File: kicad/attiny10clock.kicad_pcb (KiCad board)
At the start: 2 copper layers, 71 x 37 mm, 41 parts, among them J1 USB_B_Micro, J2 Conn_02x04_Odd_Even, SW1 SW_DIP_x01, SW2 SW_DIP_x01, SW3 SW_DIP_x01, SW4 SW_DIP_x01, SW5 SW_DIP_x01, U1 ATtiny10-TS, U2 NPIC6C595, U3 NPIC6C595, U4 NPIC6C595, U5 NPIC6C595, U6 RT8097AHGB, X1 DFA-S15

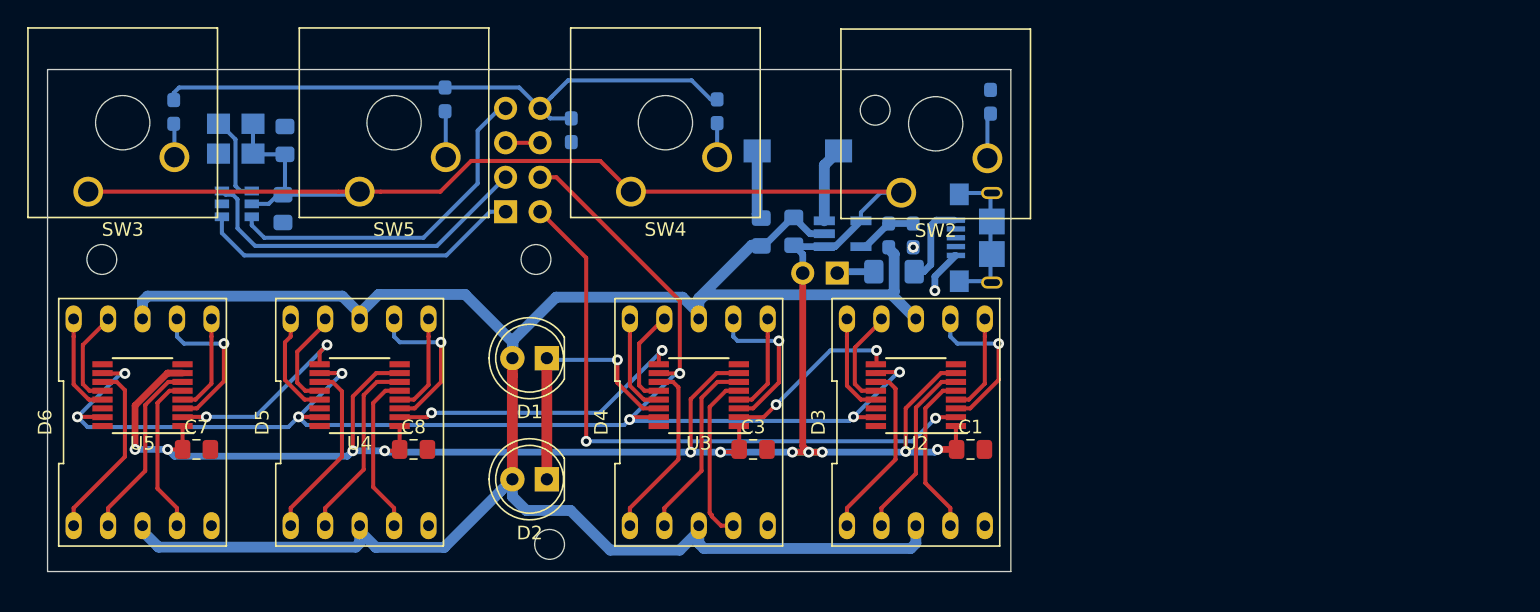
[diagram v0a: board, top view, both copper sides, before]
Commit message: Finalize rev 2 pcb
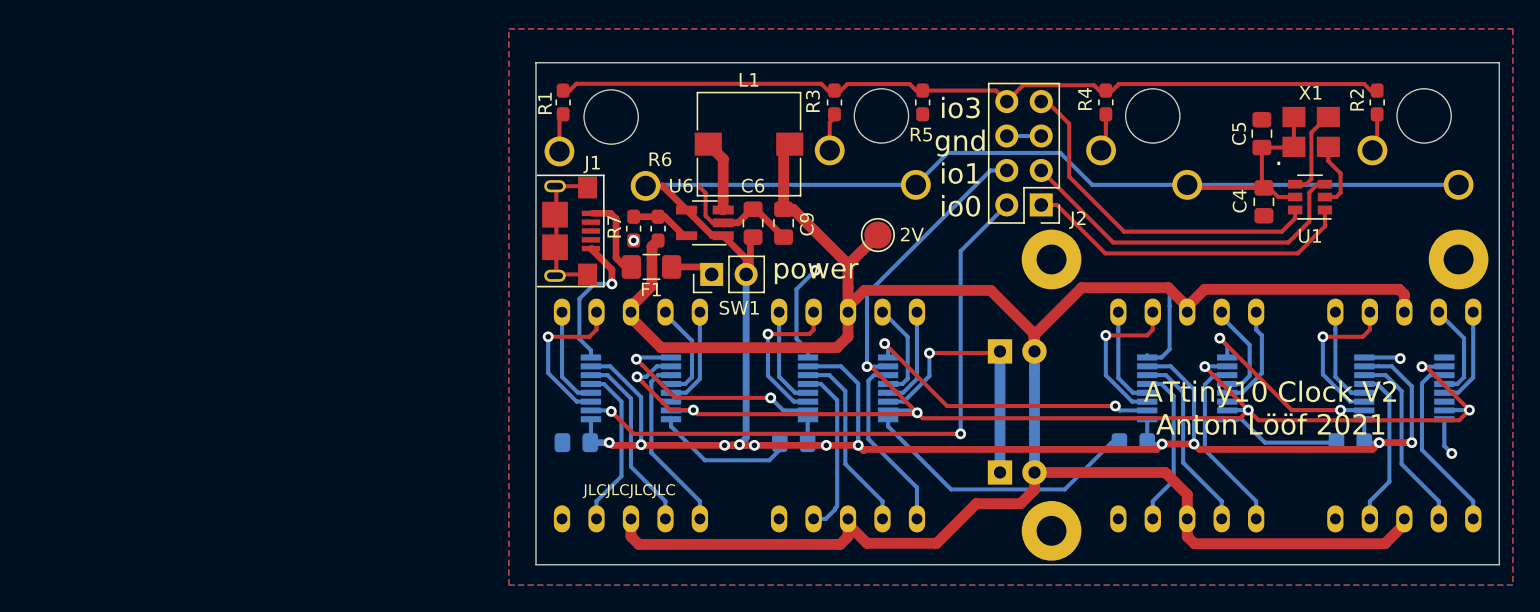
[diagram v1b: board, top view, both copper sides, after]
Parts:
- removed H3: MountingHole, MountingHole:MountingHole_2.2mm_M2
- added 2V: TestPoint, TestPoint:TestPoint_Pad_D2.0mm, F.Cu at (114.2, 100.2)
- C1, C3, C7, C8, D1, D2, D3, D4, D5, D6, SW2, SW3, SW4, SW5, U2, U3, U4, U5: moved to B.Cu
- C4, C5, C6, C9, F1, J1, J2, L1, R1, R2, R3, R4, R5, R6, R7, SW1, U1, U6, X1: moved to F.Cu
- H1, H2, H4: value MountingHole -> MountingHole_Pad; footprint MountingHole:MountingHole_2.2mm_M2 -> MountingHole:MountingHole_2.2mm_M2_Pad
- moved SW3 101.0 mm to (157.0, 96.5), turned to 0 degrees
- moved D6 93.0 mm to (153.0, 113.5), turned to 180 degrees
- moved U5 93.0 mm to (153.0, 111.5), turned to 0 degrees
- moved R2 88.7 mm to (151.0, 90.4)
- moved C7 85.1 mm to (149.0, 115.5), turned to 180 degrees
- moved X1 79.2 mm to (146.1, 92.7), turned to 0 degrees
- moved U1 79.1 mm to (146.1, 97.4), turned to 180 degrees
- moved H2 72.8 mm to (127.0, 122.0)
- moved C4 72.3 mm to (142.7, 97.8)
- moved C5 72.0 mm to (142.5, 92.7)
- moved D5 61.0 mm to (137.0, 113.5), turned to 180 degrees
- moved SW5 61.0 mm to (137.0, 96.5), turned to 0 degrees
- moved U4 61.0 mm to (137.0, 111.5), turned to 0 degrees
- moved C8 53.1 mm to (133.0, 115.5), turned to 180 degrees
- moved R4 48.7 mm to (131.0, 90.4)
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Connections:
- H1 pad 1: (no net) -> GND
- H2 pad 1: (no net) -> GND
- H4 pad 1: (no net) -> GND
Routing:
- net GND: track 12.7 -> 87.7 mm, vias 2 -> 5
- net btn_in: track 45.4 -> 62.2 mm
- net 2v: track 161.6 -> 171.6 mm
- net Net-(U2-Pad9): track 13.2 -> 16.8 mm
- net +5V: track 209.7 -> 212.5 mm
- net ser_clk: track 111.0 -> 112.5 mm
- net Net-(R4-Pad2): track 3.41 -> 2.80 mm
- net Net-(R1-Pad2): track 3.39 -> 2.85 mm
- added copper zone on B.Cu, net GND
- added copper zone on F.Cu, net GND
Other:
- board text added: "."
- board text added: "ATtiny10 Clock V2 Anton Lööf 2021"
- board text added: "JLCJLCJLCJLC"
- board text added: "io3 gnd io1 io0"
- board text added: "power"
